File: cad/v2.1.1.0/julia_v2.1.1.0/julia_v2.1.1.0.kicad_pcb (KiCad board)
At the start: 4 copper layers, 63.2 x 47.8 mm, 104 parts, among them J1 Barrel_Jack_Switch, J2 JTAG/C2/UART Header, J4 Molex 0541044031, J5 Molex 0522710679, U1 EP4CE6F17, U2 AZ1117-3.3, U3 AZ1117-2.5, U4 NCP565ST12T3G, U5 W25Q80DVSNIG, U6 EFM8BB21F16I-C-QFN20, U7 TPS61165_SOT23, U8 AS4C4M32S-7BCN, X1 50MHz

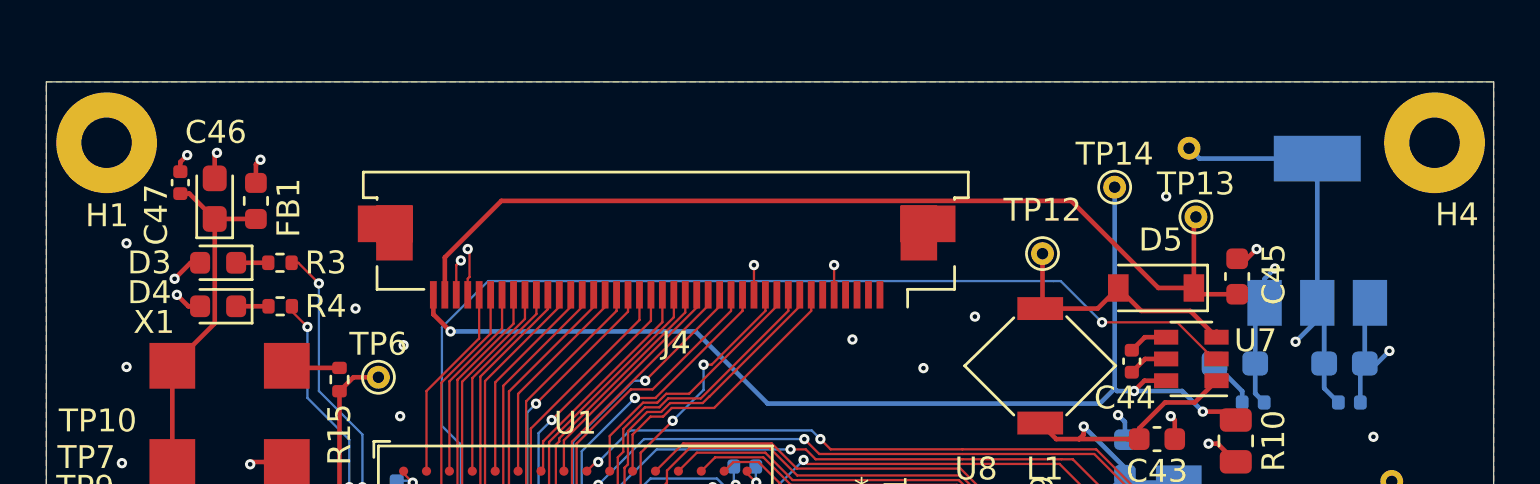
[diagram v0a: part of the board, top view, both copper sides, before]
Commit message: Updated 3d rendering
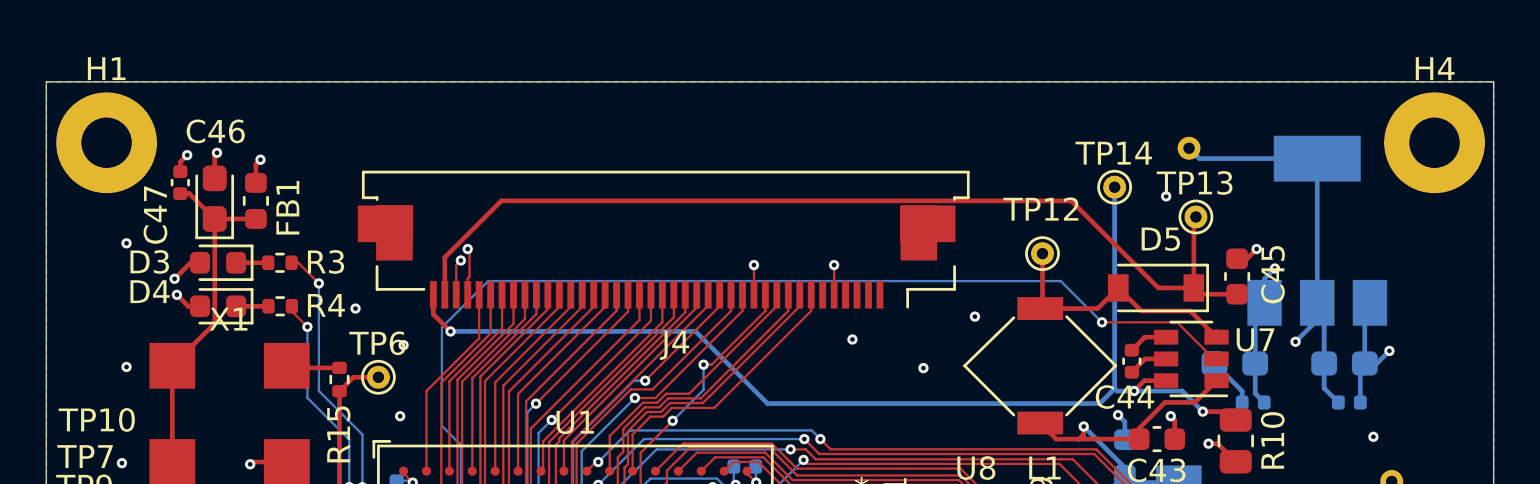
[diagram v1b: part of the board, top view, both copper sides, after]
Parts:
- H1, H2, H3, H4: footprint MountingHole:MountingHole_2.2mm_M2_Pad -> ik:MountingHole_2.2mm_M2_Pad
- X1: footprint Oscillator:Oscillator_SMD_EuroQuartz_XO91-4Pin_7.0x5.0mm -> ik:Oscillator_SMD_EuroQuartz_XO91-4Pin_7.0x5.0mm
